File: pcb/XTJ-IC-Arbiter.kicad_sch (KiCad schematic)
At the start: 41 parts, among them J3 DTM13-12PA-R008, Q1 2N7000, SW1 SW_DIP_x01, SW2 SW_DIP_x01, U1 LM2672N-5.0, U3 Teensy4.0, U4 MCP2562-H-P, U5 SP723APP

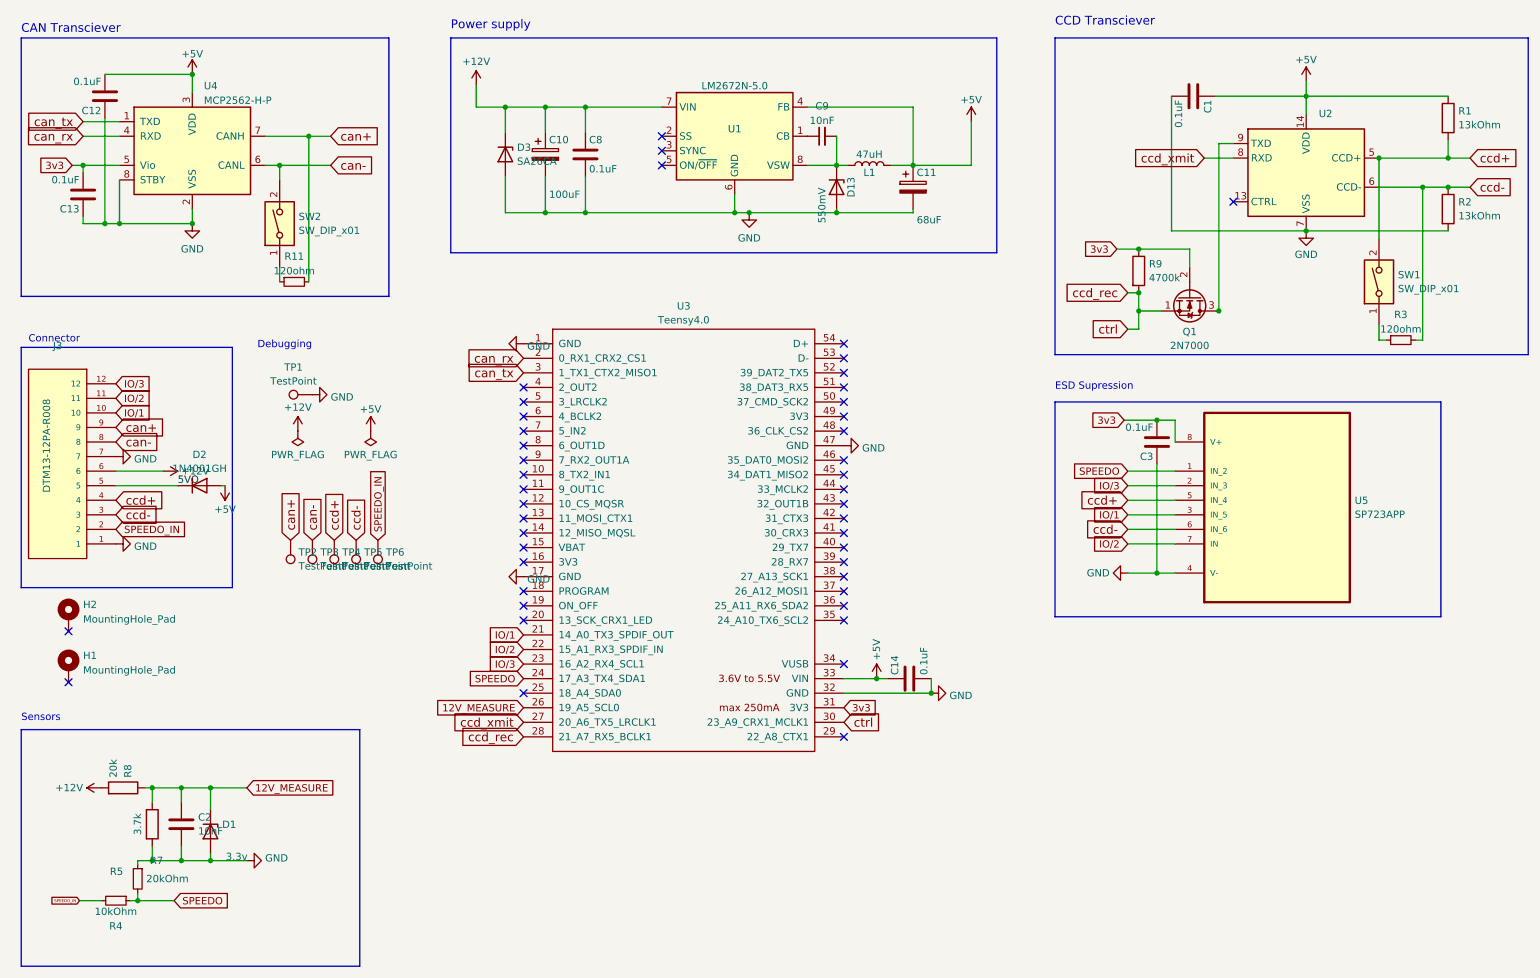
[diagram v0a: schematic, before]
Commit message: tmp
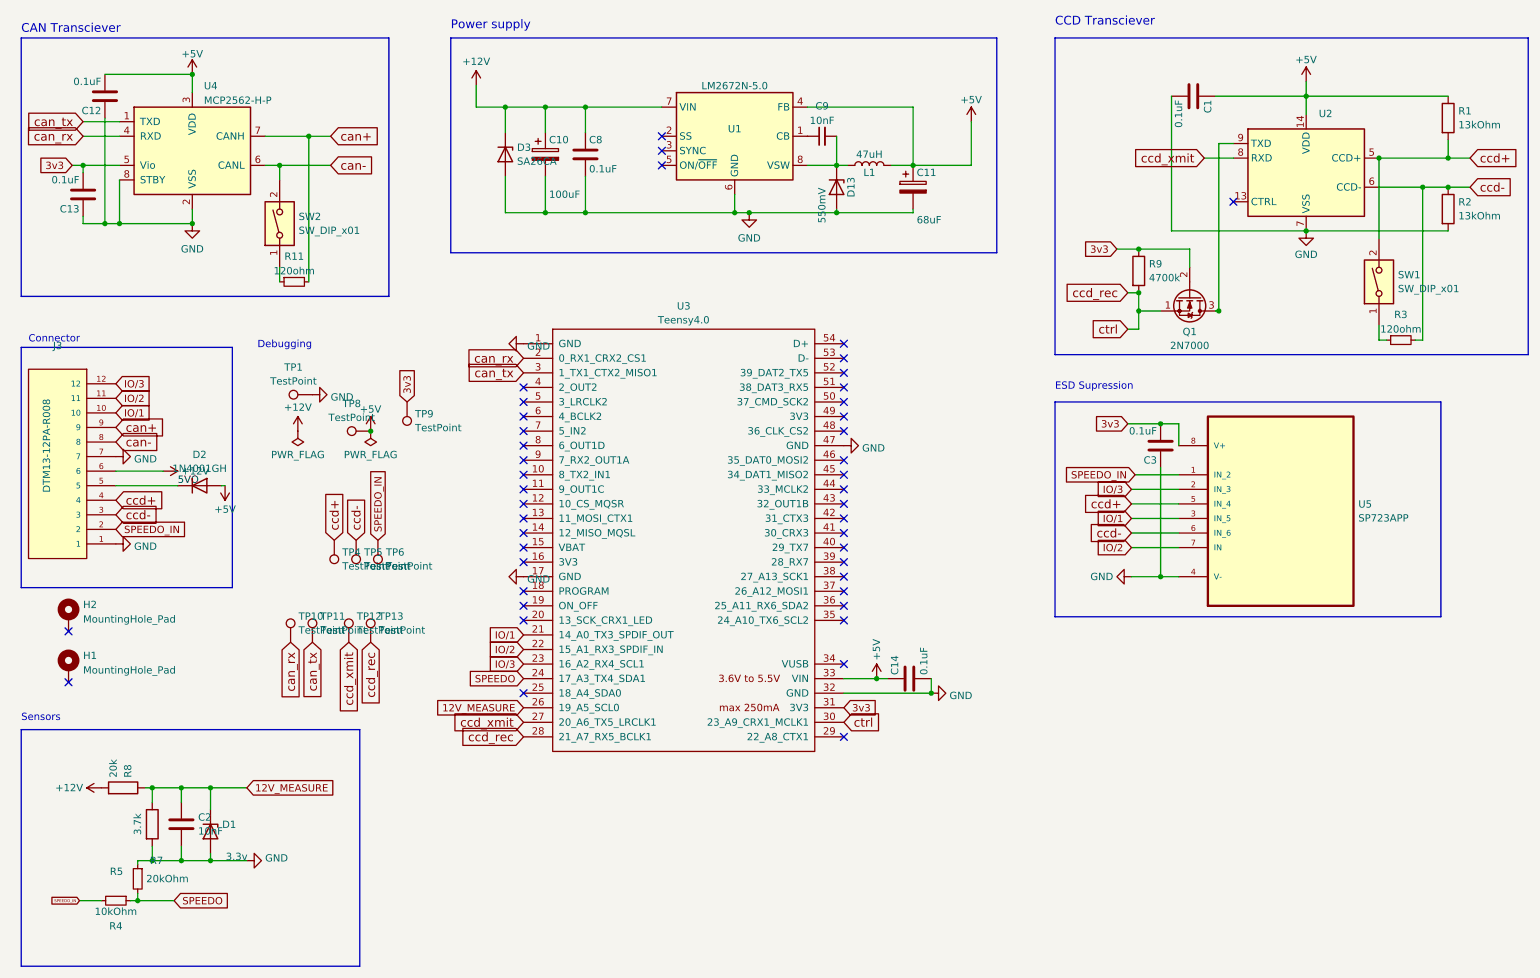
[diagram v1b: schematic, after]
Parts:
- removed TP2, TP3: TestPoint, TestPoint:TestPoint_Loop_D2.50mm_Drill1.0mm, symbol Connector:TestPoint
- added TP10, TP11, TP12, TP13, TP8, TP9: TestPoint, TestPoint:TestPoint_Loop_D2.50mm_Drill1.0mm, symbol Connector:TestPoint
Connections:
- net +5V: now also TP8.1
- net 3v3: now also TP9.1
- net SPEEDO: no longer U5.1 (IN_2)
- net SPEEDO_IN: now also U5.1 (IN_2)
- net can_rx: now also TP10.1
- net can_tx: now also TP11.1
- net ccd_rec: now also TP13.1
- net ccd_xmit: now also TP12.1
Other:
- moved on the sheet: C3, U5
